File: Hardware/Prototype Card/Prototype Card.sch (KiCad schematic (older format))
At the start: 2 parts

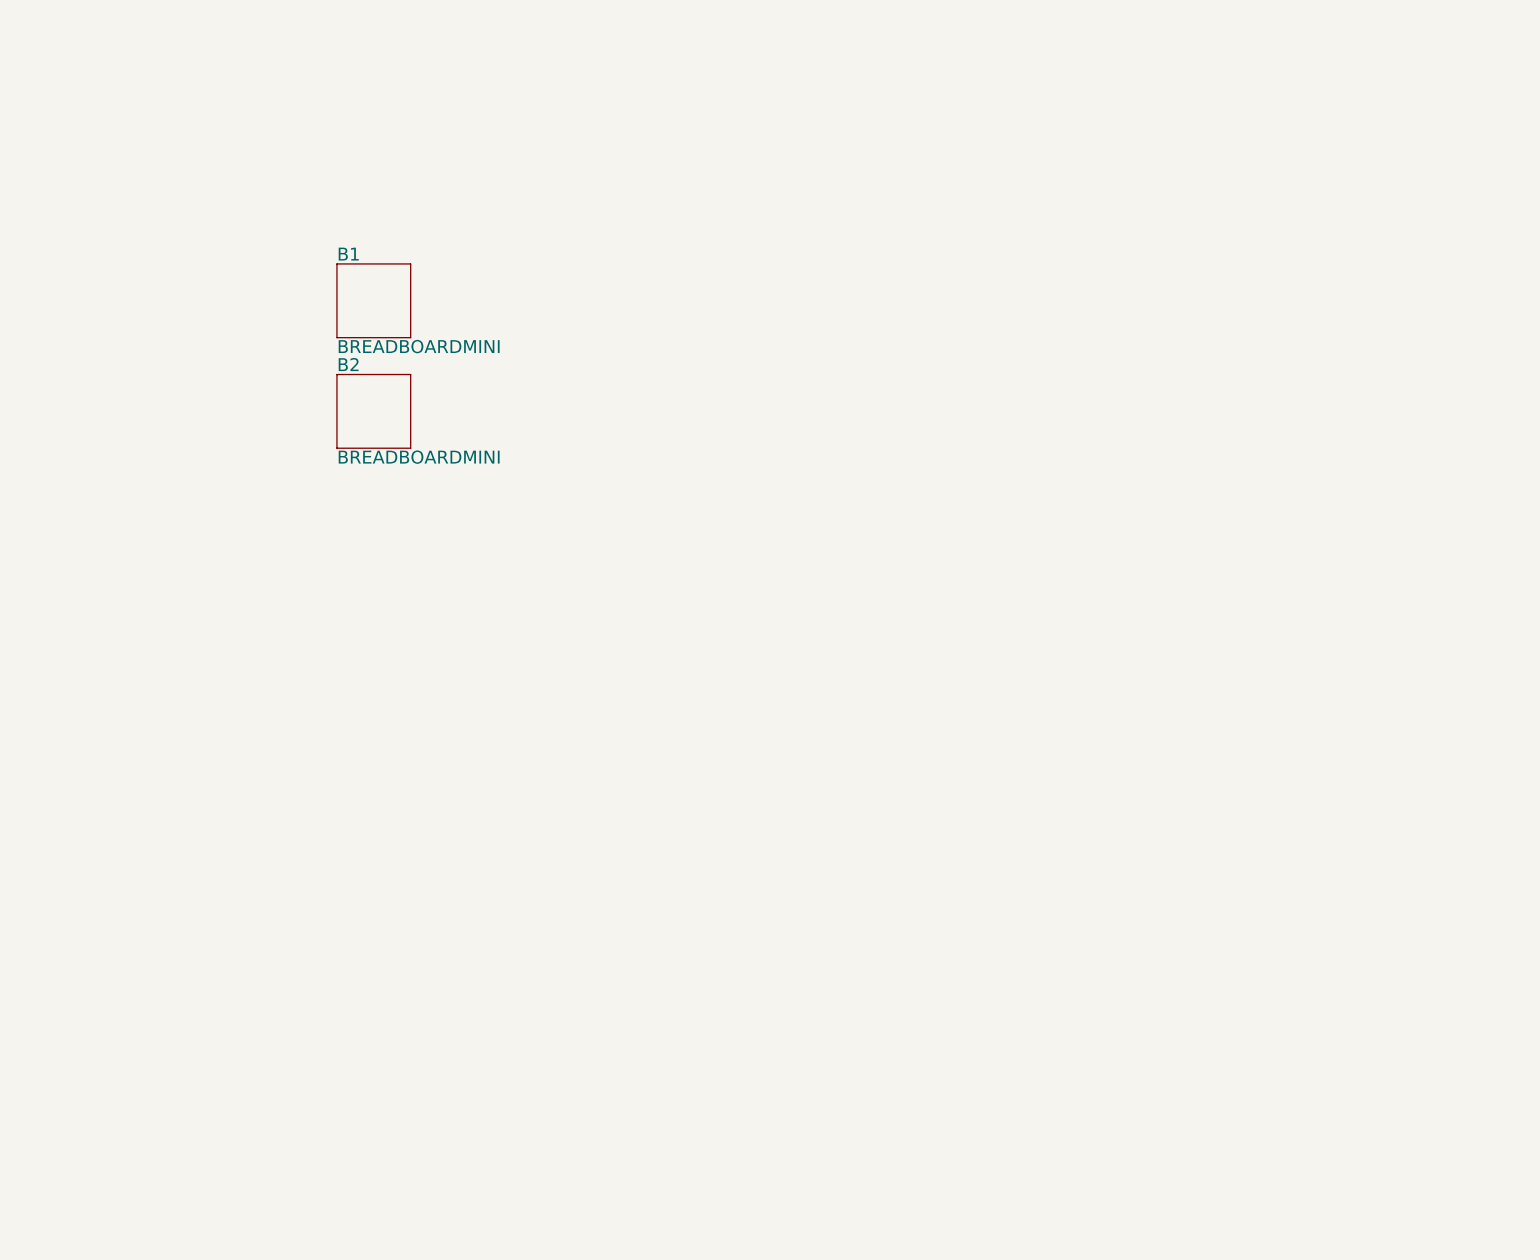
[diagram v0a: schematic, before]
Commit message: Working on schematic capture
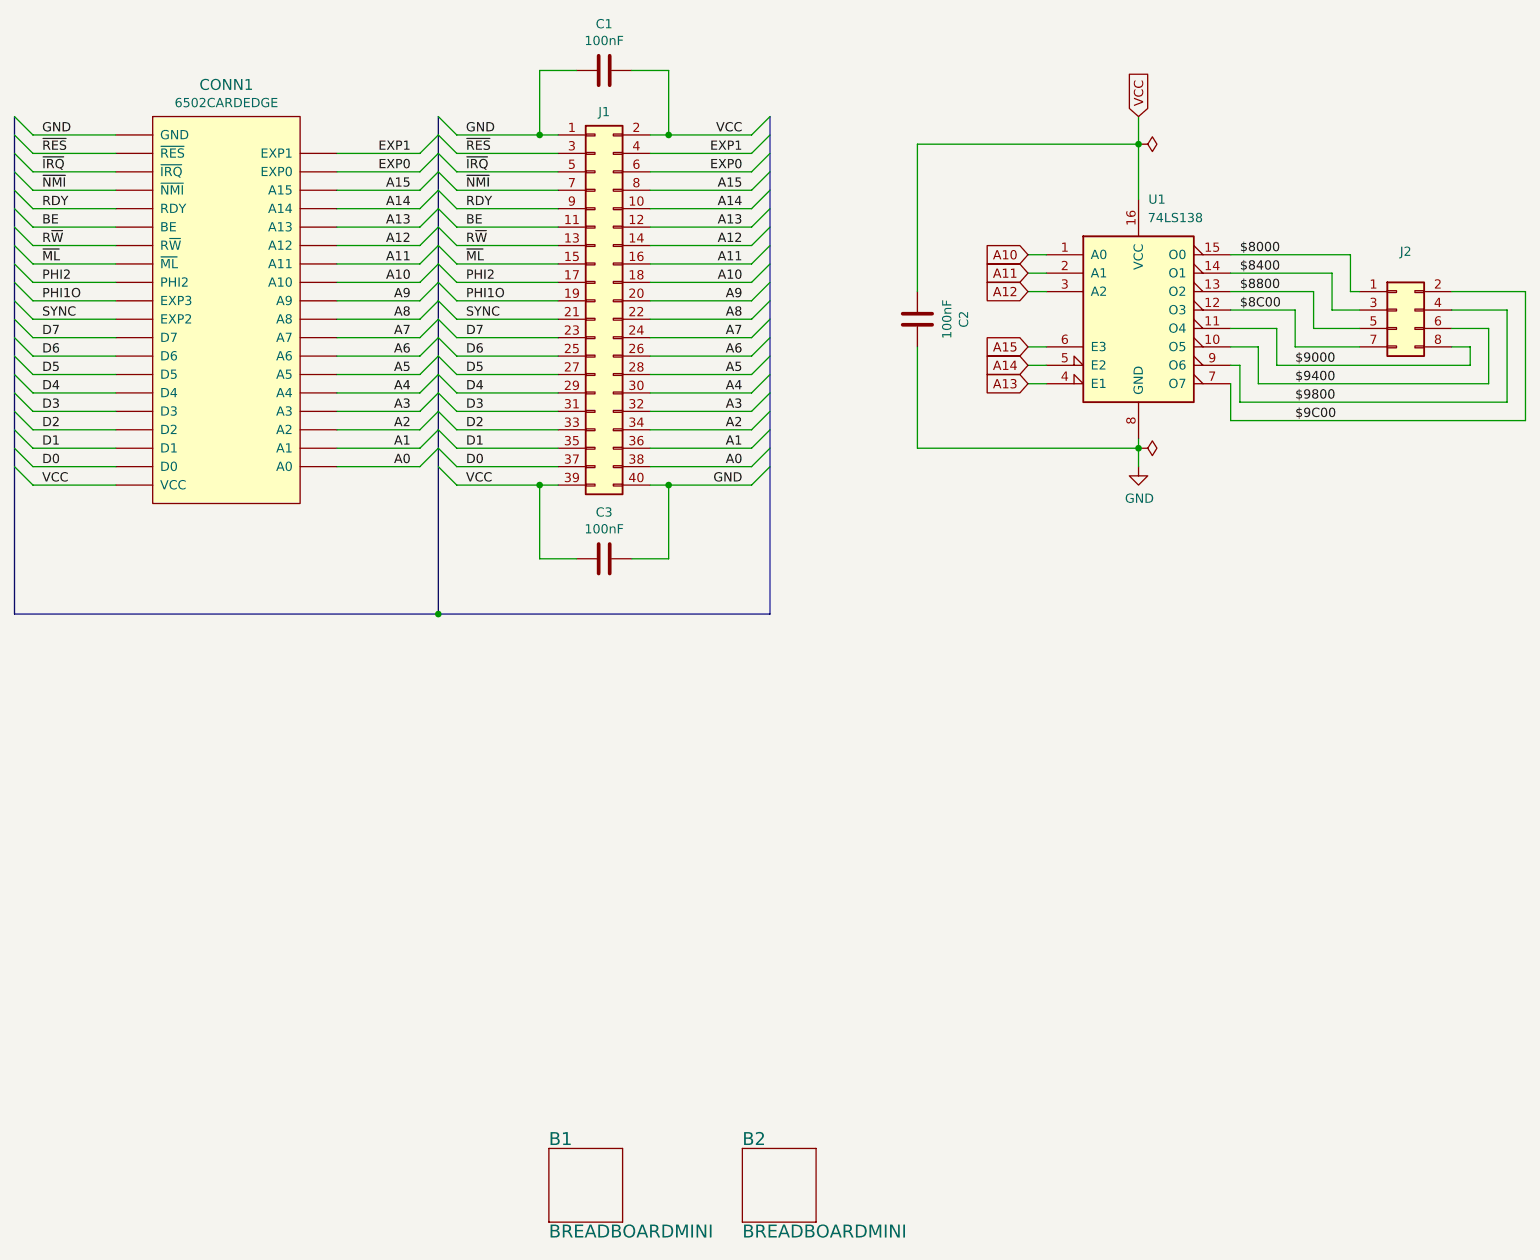
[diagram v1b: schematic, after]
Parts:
- added C1, C2, C3: 100nF, Capacitor_SMD:C_0805_2012Metric, symbol Device:C
- added CONN1: 6502CARDEDGE, Prototype Card:6502CARDEDGE, symbol Prototype_Card:6502CARDEDGE
- added J1: Conn_02x20_Odd_Even, Connector_PinHeader_2.54mm:PinHeader_2x20_P2.54mm_Vertical, symbol Connector_Generic:Conn_02x20_Odd_Even
- added J2: Conn_02x04_Odd_Even, Connector_PinHeader_2.54mm:PinHeader_2x04_P2.54mm_Vertical, symbol Connector_Generic:Conn_02x04_Odd_Even
- added U1: 74LS138, Package_SO:SOIC-16_3.9x9.9mm_P1.27mm, symbol 74xx:74LS138
- B1, B2: footprint Prototyping Card:BREADBOARD-MINI -> Prototype Card:BREADBOARD-MINI
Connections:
- new net $8000: J2.1 (Pin_1), U1.15 (O0)
- new net $8400: J2.3 (Pin_3), U1.14 (O1)
- new net $8800: J2.5 (Pin_5), U1.13 (O2)
- new net $8C00: J2.7 (Pin_7), U1.12 (O3)
- new net $9000: J2.8 (Pin_8), U1.11 (O4)
- new net $9400: J2.6 (Pin_6), U1.10 (O5)
- new net $9800: J2.4 (Pin_4), U1.9 (O6)
- new net $9C00: J2.2 (Pin_2), U1.7 (O7)
- new net A0: CONN1.A0, J1.38 (Pin_38)
- new net A1: CONN1.A1, J1.36 (Pin_36)
- new net A10: CONN1.A10, J1.18 (Pin_18), U1.1 (A0)
- new net A11: CONN1.A11, J1.16 (Pin_16), U1.2 (A1)
- new net A12: CONN1.A12, J1.14 (Pin_14), U1.3 (A2)
- new net A13: CONN1.A13, J1.12 (Pin_12), U1.4 (E1)
- new net A14: CONN1.A14, J1.10 (Pin_10), U1.5 (E2)
- new net A15: CONN1.A15, J1.8 (Pin_8), U1.6 (E3)
- new net A2: CONN1.A2, J1.34 (Pin_34)
- new net A3: CONN1.A3, J1.32 (Pin_32)
- new net A4: CONN1.A4, J1.30 (Pin_30)
- new net A5: CONN1.A5, J1.28 (Pin_28)
- new net A6: CONN1.A6, J1.26 (Pin_26)
- new net A7: CONN1.A7, J1.24 (Pin_24)
- new net A8: CONN1.A8, J1.22 (Pin_22)
- new net A9: CONN1.A9, J1.20 (Pin_20)
- new net BE: CONN1.BE, J1.11 (Pin_11)
- new net D0: CONN1.D0, J1.37 (Pin_37)
- new net D1: CONN1.D1, J1.35 (Pin_35)
- new net D2: CONN1.D2, J1.33 (Pin_33)
- new net D3: CONN1.D3, J1.31 (Pin_31)
- new net D4: CONN1.D4, J1.29 (Pin_29)
- new net D5: CONN1.D5, J1.27 (Pin_27)
- new net D6: CONN1.D6, J1.25 (Pin_25)
- new net D7: CONN1.D7, J1.23 (Pin_23)
- new net EXP0: CONN1.EXP0, J1.6 (Pin_6)
- new net EXP1: CONN1.EXP1, J1.4 (Pin_4)
- new net GND: C1.1, C2.2, C3.2, CONN1.GND, J1.1 (Pin_1), J1.40 (Pin_40), U1.8 (GND)
- new net PHI1O: CONN1.EXP3, J1.19 (Pin_19)
- new net PHI2: CONN1.PHI2, J1.17 (Pin_17)
- new net RDY: CONN1.RDY, J1.9 (Pin_9)
- new net R~W: CONN1.R~W, J1.13 (Pin_13)
- new net SYNC: CONN1.EXP2, J1.21 (Pin_21)
- new net VCC: C1.2, C2.1, C3.1, CONN1.VCC, J1.2 (Pin_2), J1.39 (Pin_39), U1.16 (VCC)
- new net ~IRQ: CONN1.~IRQ, J1.5 (Pin_5)
- new net ~ML: CONN1.~ML, J1.15 (Pin_15)
- new net ~NMI: CONN1.~NMI, J1.7 (Pin_7)
- new net ~RES: CONN1.~RES, J1.3 (Pin_3)
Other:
- moved on the sheet: B1, B2

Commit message: Generate production files
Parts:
- B1, B2: Sparkfun (none) -> PRT-12047
- C1, C2, C3: LCSC (none) -> C49678
- U1: LCSC (none) -> C5602
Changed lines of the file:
@@
 F 2 "Prototype Card:BREADBOARD-MINI" H 4350 7400 50  0001 C CNN
 F 3 "" H 4350 7400 50  0001 C CNN
+F 4 "PRT-12047" H 4350 7400 50  0001 C CNN "Sparkfun"
 	1    4350 7400
 	1    0    0    -1
@@
 F 2 "Prototype Card:BREADBOARD-MINI" H 5400 7400 50  0001 C CNN
 F 3 "" H 5400 7400 50  0001 C CNN
+F 4 "PRT-12047" H 5400 7400 50  0001 C CNN "Sparkfun"
 	1    5400 7400
 	1    0    0    -1
@@
 F 2 "Package_SO:SOIC-16_3.9x9.9mm_P1.27mm" H 7350 2650 50  0001 C CNN
 F 3 "http://www.ti.com/lit/gpn/sn74LS138" H 7350 2650 50  0001 C CNN
+F 4 "C5602" H 7350 2650 50  0001 C CNN "LCSC"
 	1    7350 2650
 	1    0    0    -1
@@
 F 2 "Capacitor_SMD:C_0805_2012Metric" H 4488 1200 50  0001 C CNN
 F 3 "~" H 4450 1350 50  0001 C CNN
+F 4 "C49678" V 4450 1350 50  0001 C CNN "LCSC"
 	1    4450 1350
 	0    -1   -1   0
@@
 F 2 "Capacitor_SMD:C_0805_2012Metric" H 4488 3850 50  0001 C CNN
 F 3 "~" H 4450 4000 50  0001 C CNN
+F 4 "C49678" H 4450 4000 50  0001 C CNN "LCSC"
 	1    4450 4000
 	0    -1   -1   0
@@
 F 2 "Capacitor_SMD:C_0805_2012Metric" H 6188 2550 50  0001 C CNN
 F 3 "~" H 6150 2700 50  0001 C CNN
+F 4 "C49678" H 6150 2700 50  0001 C CNN "LCSC"
 	1    6150 2700
 	1    0    0    -1
